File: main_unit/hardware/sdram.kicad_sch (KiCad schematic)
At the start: 1 part, among them U3 W9864G6KH-6

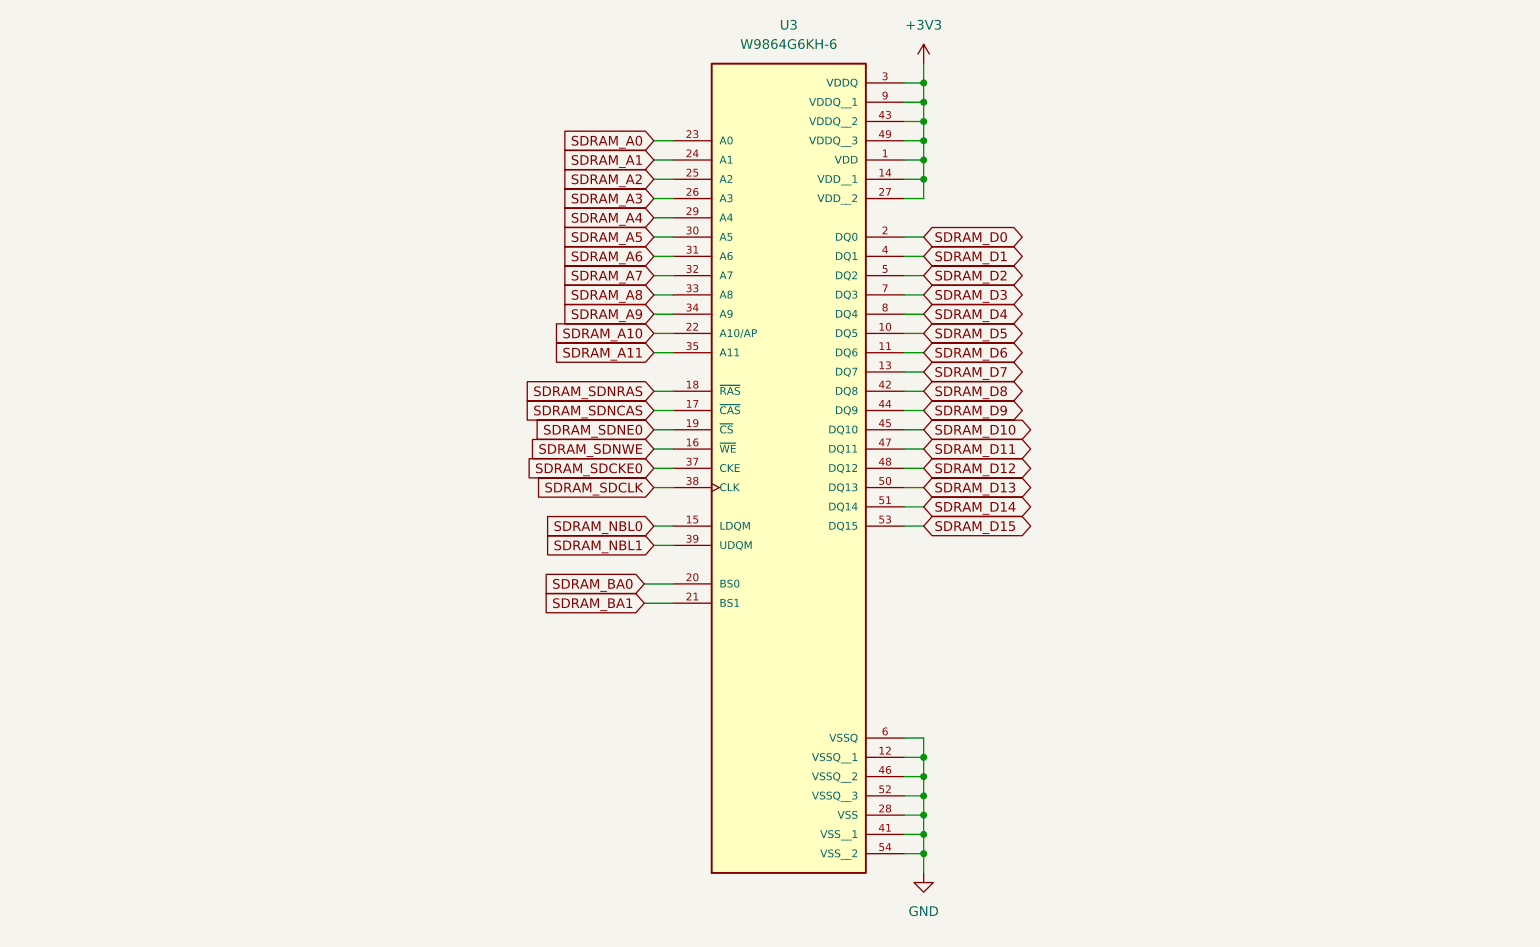
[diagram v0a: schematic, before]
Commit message: main_unit/hardware: Add in capacitors for SDRAM chip
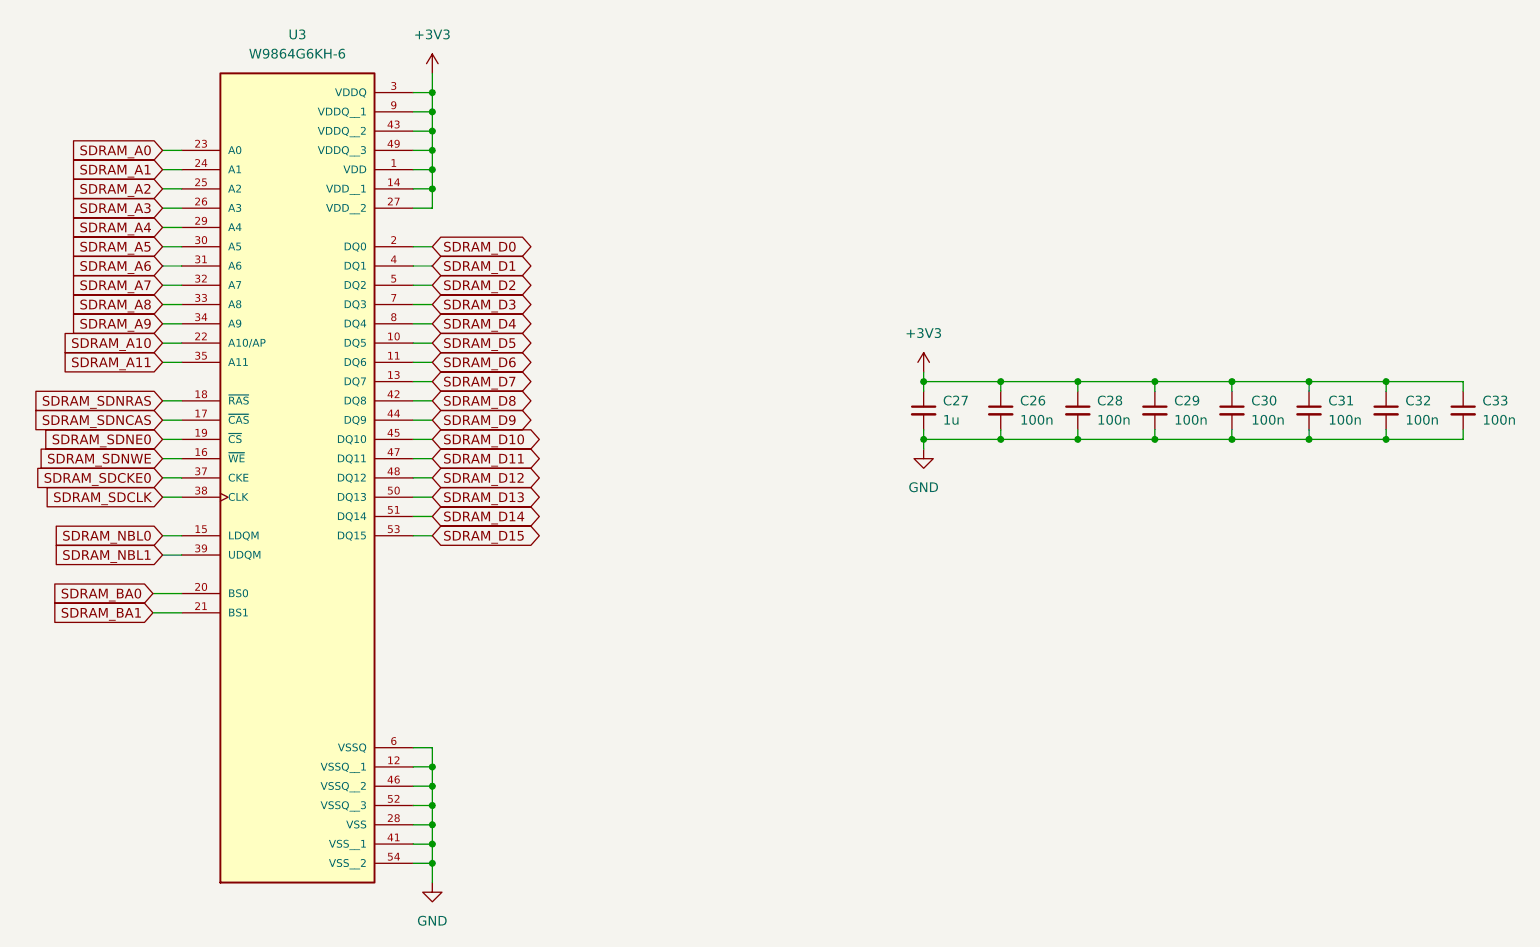
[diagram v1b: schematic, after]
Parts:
- added C26, C28, C29, C30, C31, C32, C33: 100n, Capacitor_SMD:C_0402_1005Metric, symbol Device:C_Small
- added C27: 1u, Capacitor_SMD:C_0603_1608Metric, symbol Device:C_Small
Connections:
- net +3V3: now also C26.1, C27.1, C28.1, C29.1, C30.1, C31.1, C32.1, C33.1
- net GND: now also C26.2, C27.2, C28.2, C29.2, C30.2, C31.2, C32.2, C33.2
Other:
- moved on the sheet: U3
